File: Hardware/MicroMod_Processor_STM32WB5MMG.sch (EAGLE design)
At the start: 22 parts, among them J1 MICROMOD-2222, Q1 20V/4.2A/52mΩ/1.4W, U1 STM32WB5MMG, U2 W25QXX128MBIT-6X5, U3 ESD Diode

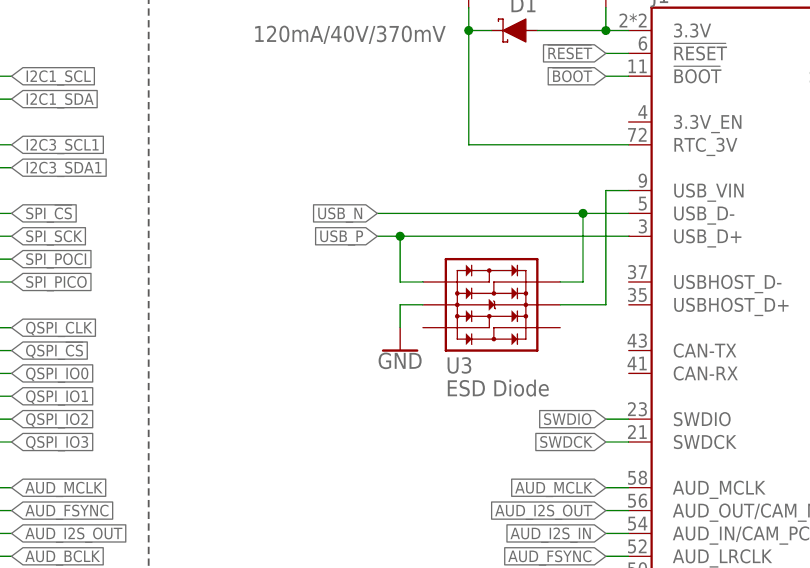
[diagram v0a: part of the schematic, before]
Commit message: v10 Update
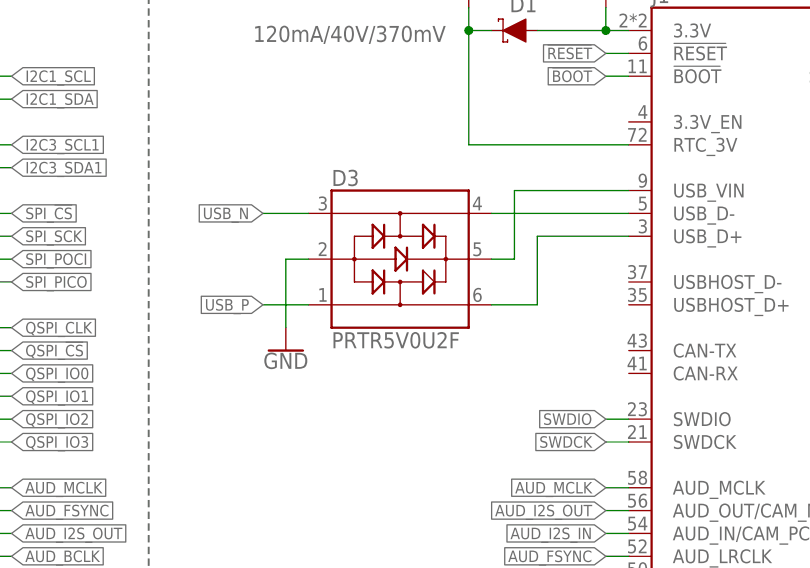
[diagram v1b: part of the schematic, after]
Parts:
- removed U3: ESD Diode, SparkFun-DiscreteSemi:TVS_DIODE_ARRAY_DT1042-04SO-7
- added D3: PRTR5V0U2F, SparkFun-IC-Power:PRTR5V0U2F
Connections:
- removed net N$2: J1.USB_VIN, U3.VCC
- new net N$4: D3.5, J1.USB_VIN
- new net USBIN_N: D3.4, J1.USB_D-
- new net USBIN_P: D3.6, J1.USB_D+
- net GND: now also D3.2; no longer U3.VSS
- net USB_N: now also D3.3; no longer J1.USB_D-, U3.IO4
- net USB_P: now also D3.1; no longer J1.USB_D+, U3.IO1
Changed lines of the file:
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@@
 <class number="0" name="default" width="0" drill="0">
 </class>
-<class number="1" name="USB_Diff" width="0.18" drill="0">
+<class number="1" name="USB_Diff" width="0.25" drill="0">
 <clearance class="0" value="0.2"/>
 <clearance class="1" value="0.2"/>
@@
 <part name="GND9" library="SparkFun-PowerSymbols" deviceset="GND" device=""/>
 <part name="GND10" library="SparkFun-PowerSymbols" deviceset="GND" device=""/>
-<part name="U3" library="SparkFun-DiscreteSemi" deviceset="TVS_DIODE_ARRAY" device="_DT1042-04SO-7" value="ESD Diode"/>
 <part name="GND11" library="SparkFun-PowerSymbols" deviceset="GND" device=""/>
+<part name="D3" library="SparkFun-IC-Power" deviceset="PRTR5V0U2" device="F"/>
 </parts>
 <sheets>
@@
 <attribute name="VALUE" x="76.2" y="40.386" size="1.778" layer="96" font="vector" align="top-center"/>
 </instance>
-<instance part="U3" gate="U1" x="157.48" y="139.7" smashed="yes" rot="R270">
-<attribute name="NAME" x="152.4" y="132.08" size="1.778" layer="95"/>
-<attribute name="VALUE" x="152.4" y="129.54" size="1.778" layer="96"/>
-</instance>
-<instance part="GND11" gate="1" x="147.32" y="134.62" smashed="yes">
-<attribute name="VALUE" x="147.32" y="134.366" size="1.778" layer="96" font="vector" align="top-center"/>
+<instance part="GND11" gate="1" x="134.62" y="134.62" smashed="yes">
+<attribute name="VALUE" x="134.62" y="134.366" size="1.778" layer="96" font="vector" align="top-center"/>
+</instance>
+<instance part="D3" gate="D1" x="147.32" y="144.78" smashed="yes" rot="MR180">
+<attribute name="NAME" x="139.7" y="154.686" size="1.778" layer="95" rot="MR180"/>
+<attribute name="VALUE" x="139.7" y="134.874" size="1.778" layer="96" rot="MR180" align="top-left"/>
 </instance>
 </instances>
@@
 <segment>
 <pinref part="GND11" gate="1" pin="GND"/>
-<pinref part="U3" gate="U1" pin="VSS"/>
-<wire x1="147.32" y1="137.16" x2="147.32" y2="139.7" width="0.1524" layer="91"/>
-<wire x1="147.32" y1="139.7" x2="149.86" y2="139.7" width="0.1524" layer="91"/>
+<pinref part="D3" gate="D1" pin="2"/>
+<wire x1="134.62" y1="137.16" x2="134.62" y2="144.78" width="0.1524" layer="91"/>
+<wire x1="134.62" y1="144.78" x2="137.16" y2="144.78" width="0.1524" layer="91"/>
 </segment>
 </net>
@@
 </segment>
 <segment>
-<pinref part="J1" gate="J1" pin="USB_D-"/>
-<wire x1="172.72" y1="149.86" x2="167.64" y2="149.86" width="0.1524" layer="91"/>
-<label x="144.78" y="149.86" size="1.27" layer="95" font="vector" rot="R180" xref="yes"/>
-<pinref part="U3" gate="U1" pin="IO4"/>
-<wire x1="167.64" y1="149.86" x2="144.78" y2="149.86" width="0.1524" layer="91"/>
-<wire x1="165.1" y1="142.24" x2="167.64" y2="142.24" width="0.1524" layer="91"/>
-<wire x1="167.64" y1="142.24" x2="167.64" y2="149.86" width="0.1524" layer="91"/>
-<junction x="167.64" y="149.86"/>
+<label x="132.08" y="149.86" size="1.27" layer="95" font="vector" rot="R180" xref="yes"/>
+<wire x1="137.16" y1="149.86" x2="132.08" y2="149.86" width="0.1524" layer="91"/>
+<pinref part="D3" gate="D1" pin="3"/>
 </segment>
 </net>
@@
 </segment>
 <segment>
-<pinref part="J1" gate="J1" pin="USB_D+"/>
-<label x="144.78" y="147.32" size="1.27" layer="95" font="vector" rot="R180" xref="yes"/>
-<wire x1="144.78" y1="147.32" x2="147.32" y2="147.32" width="0.1524" layer="91"/>
-<pinref part="U3" gate="U1" pin="IO1"/>
-<wire x1="147.32" y1="147.32" x2="172.72" y2="147.32" width="0.1524" layer="91"/>
-<wire x1="149.86" y1="142.24" x2="147.32" y2="142.24" width="0.1524" layer="91"/>
-<wire x1="147.32" y1="142.24" x2="147.32" y2="147.32" width="0.1524" layer="91"/>
-<junction x="147.32" y="147.32"/>
+<label x="132.08" y="139.7" size="1.27" layer="95" font="vector" rot="R180" xref="yes"/>
+<wire x1="132.08" y1="139.7" x2="137.16" y2="139.7" width="0.1524" layer="91"/>
+<pinref part="D3" gate="D1" pin="1"/>
 </segment>
 </net>
@@
 </segment>
 </net>
-<net name="N$2" class="0">
+<net name="USBIN_N" class="1">
+<segment>
+<pinref part="D3" gate="D1" pin="4"/>
+<pinref part="J1" gate="J1" pin="USB_D-"/>
+<wire x1="157.48" y1="149.86" x2="172.72" y2="149.86" width="0.1524" layer="91"/>
+</segment>
+</net>
+<net name="USBIN_P" class="1">
+<segment>
+<pinref part="D3" gate="D1" pin="6"/>
+<wire x1="157.48" y1="139.7" x2="162.56" y2="139.7" width="0.1524" layer="91"/>
+<wire x1="162.56" y1="139.7" x2="162.56" y2="147.32" width="0.1524" layer="91"/>
+<pinref part="J1" gate="J1" pin="USB_D+"/>
+<wire x1="162.56" y1="147.32" x2="172.72" y2="147.32" width="0.1524" layer="91"/>
+</segment>
+</net>
+<net name="N$4" class="0">
 <segment>
 <pinref part="J1" gate="J1" pin="USB_VIN"/>
-<wire x1="172.72" y1="152.4" x2="170.18" y2="152.4" width="0.1524" layer="91"/>
-<pinref part="U3" gate="U1" pin="VCC"/>
-<wire x1="165.1" y1="139.7" x2="170.18" y2="139.7" width="0.1524" layer="91"/>
-<wire x1="170.18" y1="139.7" x2="170.18" y2="152.4" width="0.1524" layer="91"/>
-</segment>
-</net>
+<wire x1="172.72" y1="152.4" x2="160.02" y2="152.4" width="0.1524" layer="91"/>
+<wire x1="160.02" y1="152.4" x2="160.02" y2="144.78" width="0.1524" layer="91"/>
+<pinref part="D3" gate="D1" pin="5"/>
+<wire x1="160.02" y1="144.78" x2="157.48" y2="144.78" width="0.1524" layer="91"/>
+</segment>
+</net>
